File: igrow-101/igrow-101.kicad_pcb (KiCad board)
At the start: 2 copper layers, 49.8 x 39.5 mm, 32 parts, among them P1 CONN_02X05, P2 CONN_01X01, P3 CONN_01X01, P4 CONN_01X01, P5 CONN_01X01, Q1 NPN, Q2 NPN, Q3 NPN, SW1 SW_PUSH, U1 NRF51822-MODULE, U2 SHT21

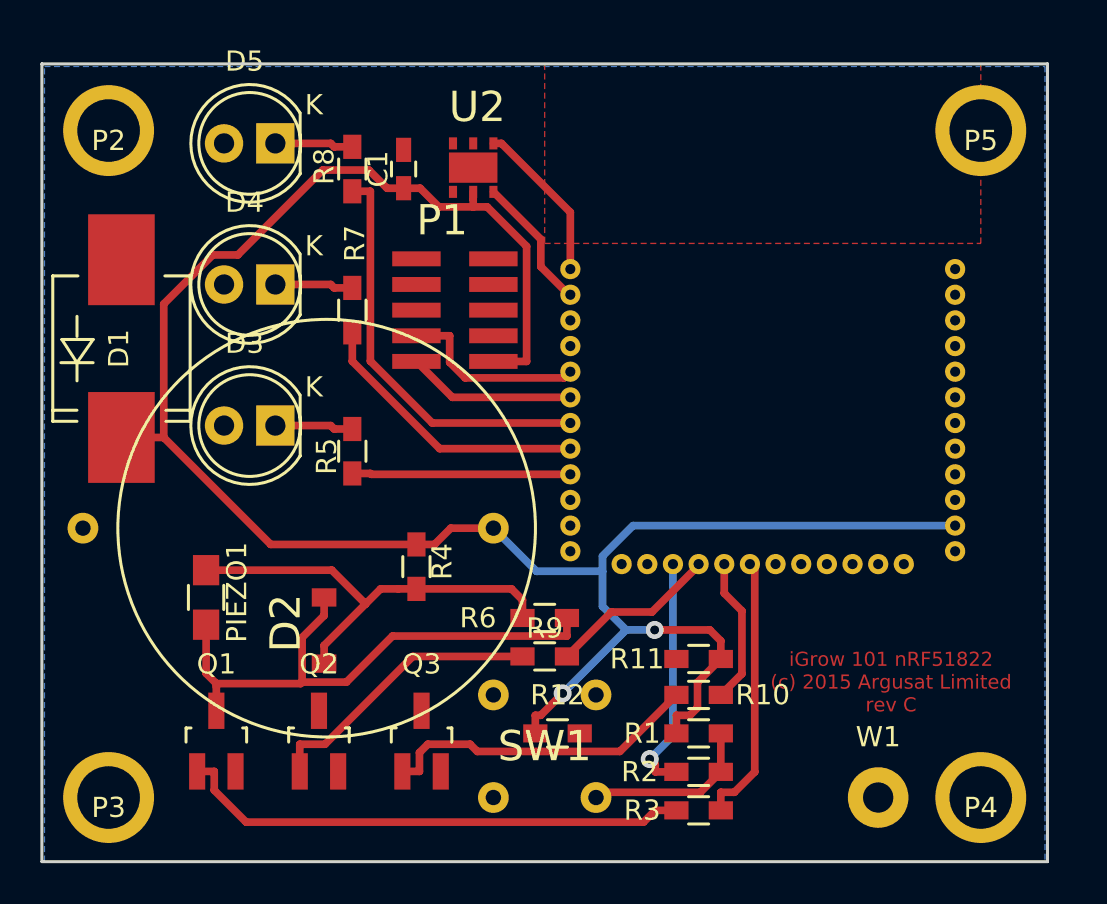
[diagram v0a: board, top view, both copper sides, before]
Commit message: Revision D as sent to dirtypcbs for fab
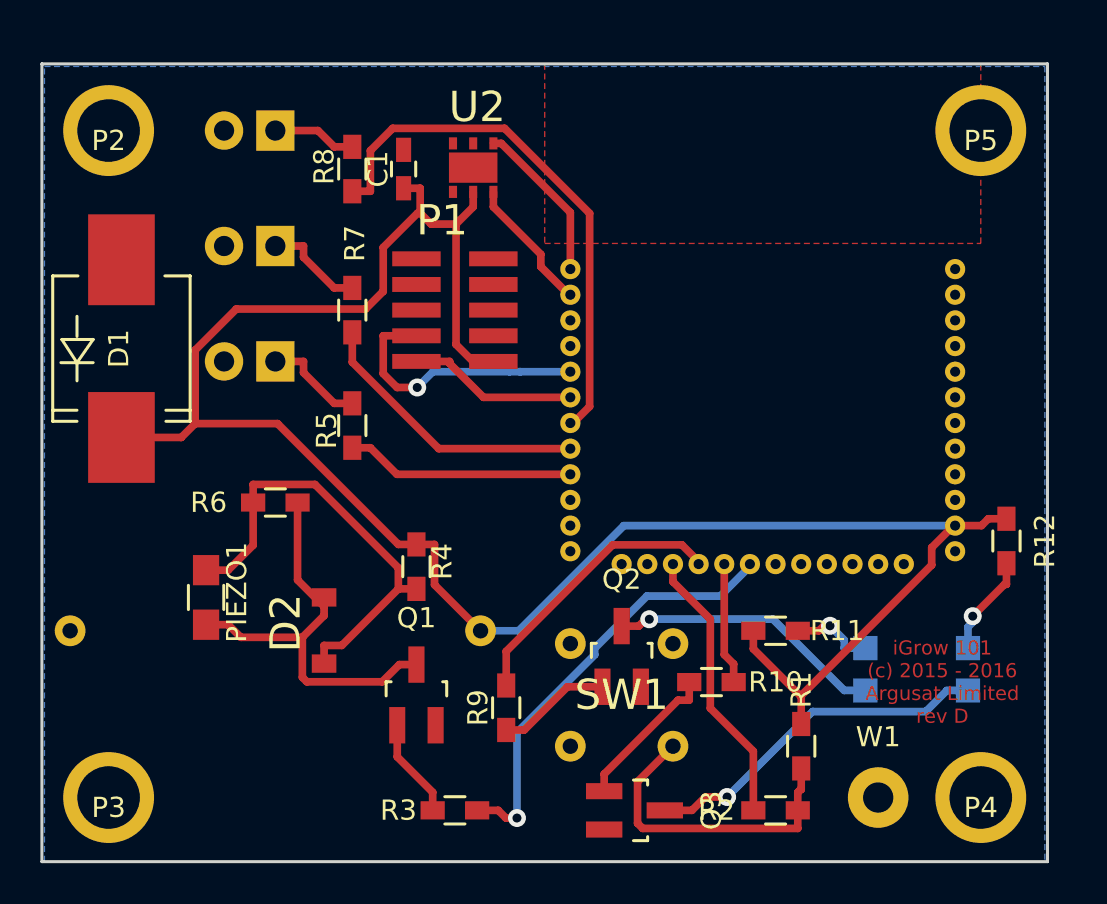
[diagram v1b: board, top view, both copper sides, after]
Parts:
- added D6: LED, LEDs:LED_0805, B.Cu at (172.1, 123.2)
- added D7: LED, LEDs:LED_0805, B.Cu at (177.2, 123.2)
- BT1, D3, D4, D5: moved to B.Cu
- moved R12 24.2 mm to (179.1, 116.8), turned to 270 degrees
- moved Q2 15.6 mm to (160.0, 122.6)
- moved R6 14.5 mm to (142.9, 114.9)
- moved R3 12.1 mm to (151.8, 130.2)
- moved Q3 11.1 mm to (160.7, 130.2), turned to 270 degrees
- moved Q1 10.2 mm to (149.9, 124.5)
- moved BT1 5.12 mm to (153.0, 121.3), turned to 90 degrees
- moved R1 5.12 mm to (168.9, 127.0), turned to 270 degrees
- moved SW1 4.58 mm to (162.6, 127.0)
- moved R2 4.26 mm to (167.6, 130.2)
- moved R11 4.06 mm to (167.6, 121.3), turned to 0 degrees
- moved D3 3.17 mm to (142.9, 108.0)
- moved R9 3.17 mm to (154.3, 125.1), turned to 90 degrees
- moved D4 1.91 mm to (142.9, 102.2)
- moved R5 1.27 mm to (146.7, 111.1)
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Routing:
- net Net-(Q1-Pad2): track 25.6 -> 4.94 mm
- net Net-(D7-Pad2): track 0.00 -> 17.5 mm, vias 0 -> 1
- net Net-(D6-Pad2): track 0.00 -> 13.7 mm, vias 0 -> 1
- net Net-(Q2-Pad2): track 14.2 -> 5.65 mm
- net Net-(Q3-Pad2): track 16.0 -> 7.47 mm
- net Net-(R3-Pad2): track 13.4 -> 21.6 mm, vias 0 -> 1
- net Net-(D2-Pad1): track 28.3 -> 21.2 mm
- net Net-(R1-Pad2): track 8.61 -> 15.6 mm
- net Net-(R8-Pad1): track 20.5 -> 26.8 mm
- net Net-(R9-Pad2): track 8.45 -> 13.9 mm
- net Net-(D7-Pad1): track 0.00 -> 5.04 mm, vias 0 -> 1
- net Net-(D6-Pad1): track 0.00 -> 4.14 mm, vias 0 -> 1
- net Net-(P1-Pad4): track 9.38 -> 13.4 mm, vias 0 -> 1
- net VCC: track 104.4 -> 102.1 mm, vias 2 -> 0
- net Net-(R2-Pad1): track 11.9 -> 13.8 mm, vias 1 -> 0
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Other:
- board text added: "iGrow 101 (c) 2015 - 2016 Argusat Limited rev D"
- board text removed: "iGrow 101 nRF51822 (c) 2015 Argusat Limited rev C"
